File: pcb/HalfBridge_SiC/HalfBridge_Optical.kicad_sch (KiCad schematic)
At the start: 18 parts, among them J3 AFBR-2624Z, J4 AFBR-2624Z, J5 AFBR-2624Z

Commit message: backplane + external lib
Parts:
- C32, C33, C34: footprint Capacitor_SMD:C_0603_1608Metric_Pad1.08x0.95mm_HandSolder -> (none)
- C35, C36, C37, C38, C39, C40: footprint Capacitor_SMD:C_0805_2012Metric_Pad1.18x1.45mm_HandSolder -> (none)
- J3, J4, J5: footprint OptoDevice:Broadcom_AFBR-16xxZ_Horizontal -> (none)
- L4, L5, L6: footprint Inductor_SMD:L_0603_1608Metric_Pad1.05x0.95mm_HandSolder -> (none)
- R27, R28, R29: footprint Resistor_SMD:R_0603_1608Metric_Pad0.98x0.95mm_HandSolder -> (none)
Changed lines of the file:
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@@
 			)
 		)
-		(property "Footprint" "Capacitor_SMD:C_0805_2012Metric_Pad1.18x1.45mm_HandSolder"
+		(property "Footprint" ""
 			(at 87.3252 100.33 0)
 			(effects
@@
 			)
 		)
-		(property "Footprint" "Inductor_SMD:L_0603_1608Metric_Pad1.05x0.95mm_HandSolder"
+		(property "Footprint" ""
 			(at 95.25 53.34 0)
 			(effects
@@
 			)
 		)
-		(property "Footprint" "Capacitor_SMD:C_0805_2012Metric_Pad1.18x1.45mm_HandSolder"
+		(property "Footprint" ""
 			(at 102.5652 60.96 0)
 			(effects
@@
 			)
 		)
-		(property "Footprint" "Capacitor_SMD:C_0805_2012Metric_Pad1.18x1.45mm_HandSolder"
+		(property "Footprint" ""
 			(at 102.5652 138.43 0)
 			(effects
@@
 			)
 		)
-		(property "Footprint" "Capacitor_SMD:C_0805_2012Metric_Pad1.18x1.45mm_HandSolder"
+		(property "Footprint" ""
 			(at 87.3252 60.96 0)
 			(effects
@@
 			)
 		)
-		(property "Footprint" "Resistor_SMD:R_0603_1608Metric_Pad0.98x0.95mm_HandSolder"
+		(property "Footprint" ""
 			(at 77.47 71.882 90)
 			(effects
@@
 			)
 		)
-		(property "Footprint" "Resistor_SMD:R_0603_1608Metric_Pad0.98x0.95mm_HandSolder"
+		(property "Footprint" ""
 			(at 77.47 107.442 90)
 			(effects
@@
 			)
 		)
-		(property "Footprint" "Resistor_SMD:R_0603_1608Metric_Pad0.98x0.95mm_HandSolder"
+		(property "Footprint" ""
 			(at 77.47 145.542 90)
 			(effects
@@
 			)
 		)
-		(property "Footprint" "Capacitor_SMD:C_0603_1608Metric_Pad1.08x0.95mm_HandSolder"
+		(property "Footprint" ""
 			(at 77.1652 138.43 0)
 			(effects
@@
 			)
 		)
-		(property "Footprint" "Capacitor_SMD:C_0603_1608Metric_Pad1.08x0.95mm_HandSolder"
+		(property "Footprint" ""
 			(at 77.1652 60.96 0)
 			(effects
@@
 			)
 		)
-		(property "Footprint" "Capacitor_SMD:C_0805_2012Metric_Pad1.18x1.45mm_HandSolder"
+		(property "Footprint" ""
 			(at 102.5652 100.33 0)
 			(effects
@@
 			)
 		)
-		(property "Footprint" "Capacitor_SMD:C_0805_2012Metric_Pad1.18x1.45mm_HandSolder"
+		(property "Footprint" ""
 			(at 87.3252 138.43 0)
 			(effects
@@
 			)
 		)
-		(property "Footprint" "OptoDevice:Broadcom_AFBR-16xxZ_Horizontal"
+		(property "Footprint" ""
 			(at 55.88 121.92 0)
 			(effects
@@
 			)
 		)
-		(property "Footprint" "OptoDevice:Broadcom_AFBR-16xxZ_Horizontal"
+		(property "Footprint" ""
 			(at 55.88 160.02 0)
 			(effects
@@
 			)
 		)
-		(property "Footprint" "Inductor_SMD:L_0603_1608Metric_Pad1.05x0.95mm_HandSolder"
+		(property "Footprint" ""
 			(at 95.25 92.71 0)
 			(effects
@@
 			)
 		)
-		(property "Footprint" "Inductor_SMD:L_0603_1608Metric_Pad1.05x0.95mm_HandSolder"
+		(property "Footprint" ""
 			(at 95.25 130.81 0)
 			(effects
@@
 			)
 		)
-		(property "Footprint" "Capacitor_SMD:C_0603_1608Metric_Pad1.08x0.95mm_HandSolder"
+		(property "Footprint" ""
 			(at 77.1652 100.33 0)
 			(effects
@@
 			)
 		)
-		(property "Footprint" "OptoDevice:Broadcom_AFBR-16xxZ_Horizontal"
+		(property "Footprint" ""
 			(at 55.88 86.36 0)
 			(effects

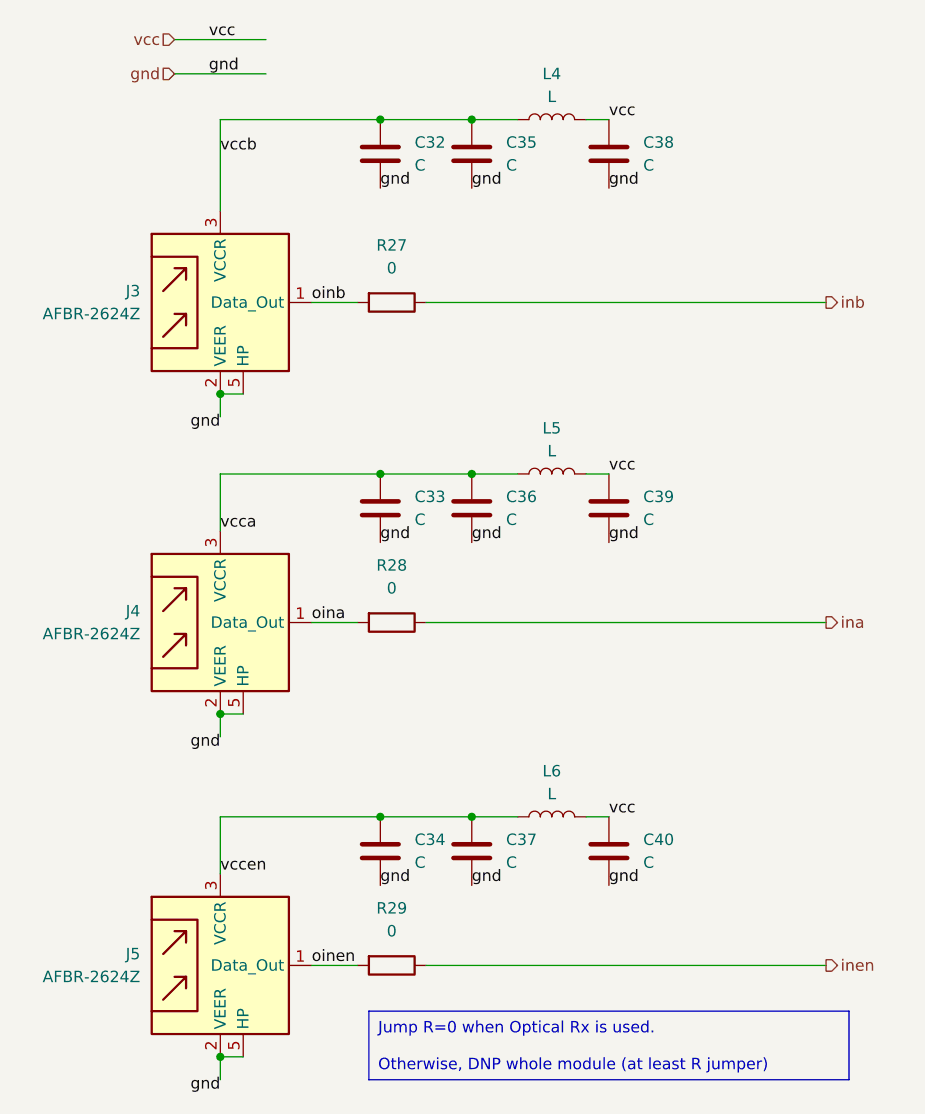
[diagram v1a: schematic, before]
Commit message: update lib
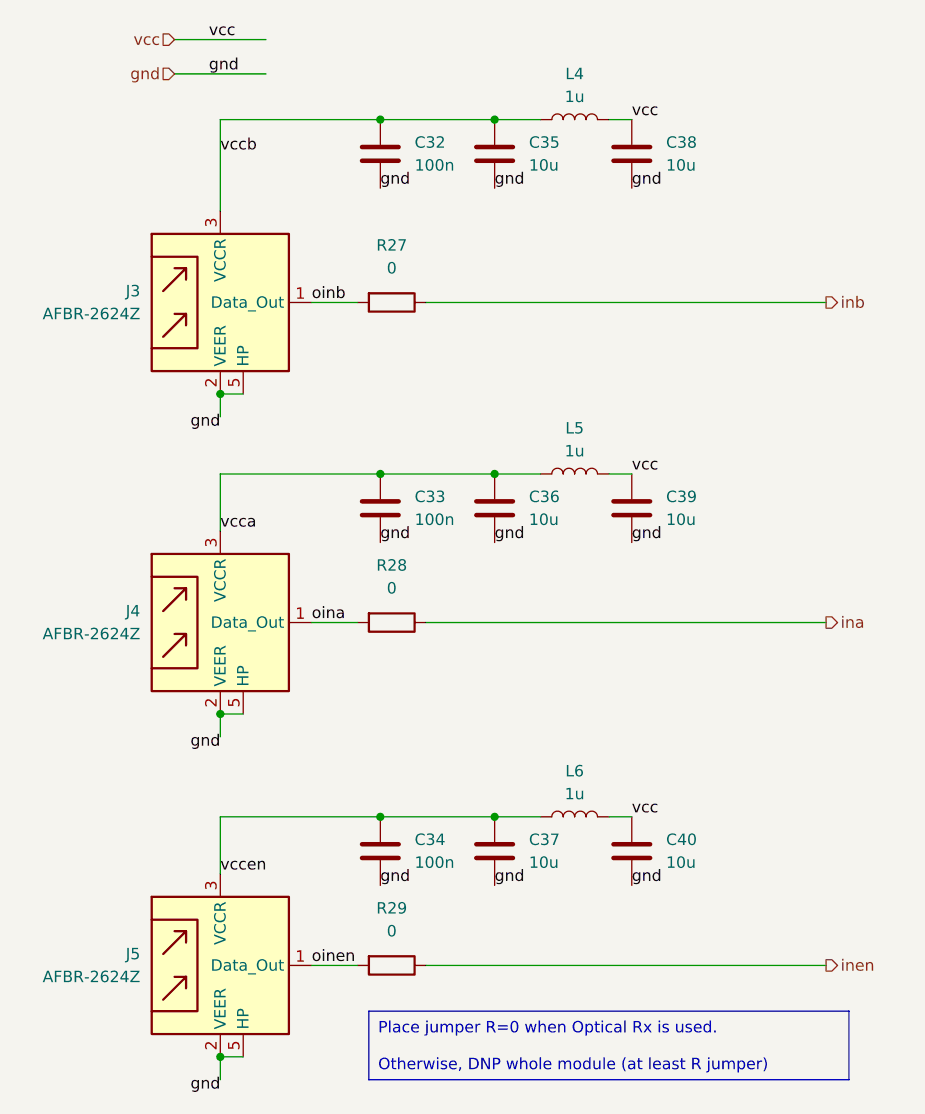
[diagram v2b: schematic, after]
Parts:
- C32, C33, C34: value C -> 100n; footprint (none) -> Capacitor_SMD:C_0603_1608Metric_Pad1.08x0.95mm_HandSolder
- C35, C36, C37, C38, C39, C40: value C -> 10u; footprint (none) -> Capacitor_SMD:C_0805_2012Metric_Pad1.18x1.45mm_HandSolder
- J3, J4, J5: footprint (none) -> OptoDevice:Broadcom_AFBR-16xxZ_Horizontal
- L4, L5, L6: value L -> 1u; footprint (none) -> Inductor_SMD:L_0603_1608Metric_Pad1.05x0.95mm_HandSolder
- R27, R28, R29: footprint (none) -> Resistor_SMD:R_0603_1608Metric_Pad0.98x0.95mm_HandSolder
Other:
- moved on the sheet: C35, C36, C37, C38, C39, C40, L4, L5, L6
